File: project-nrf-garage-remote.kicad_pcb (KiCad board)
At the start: 2 copper layers, 34.5 x 27 mm, 9 parts, among them J1 Screw_Terminal_01x02, J2 Screw_Terminal_01x04, Q1 BSS138W, Q2 BSS138W

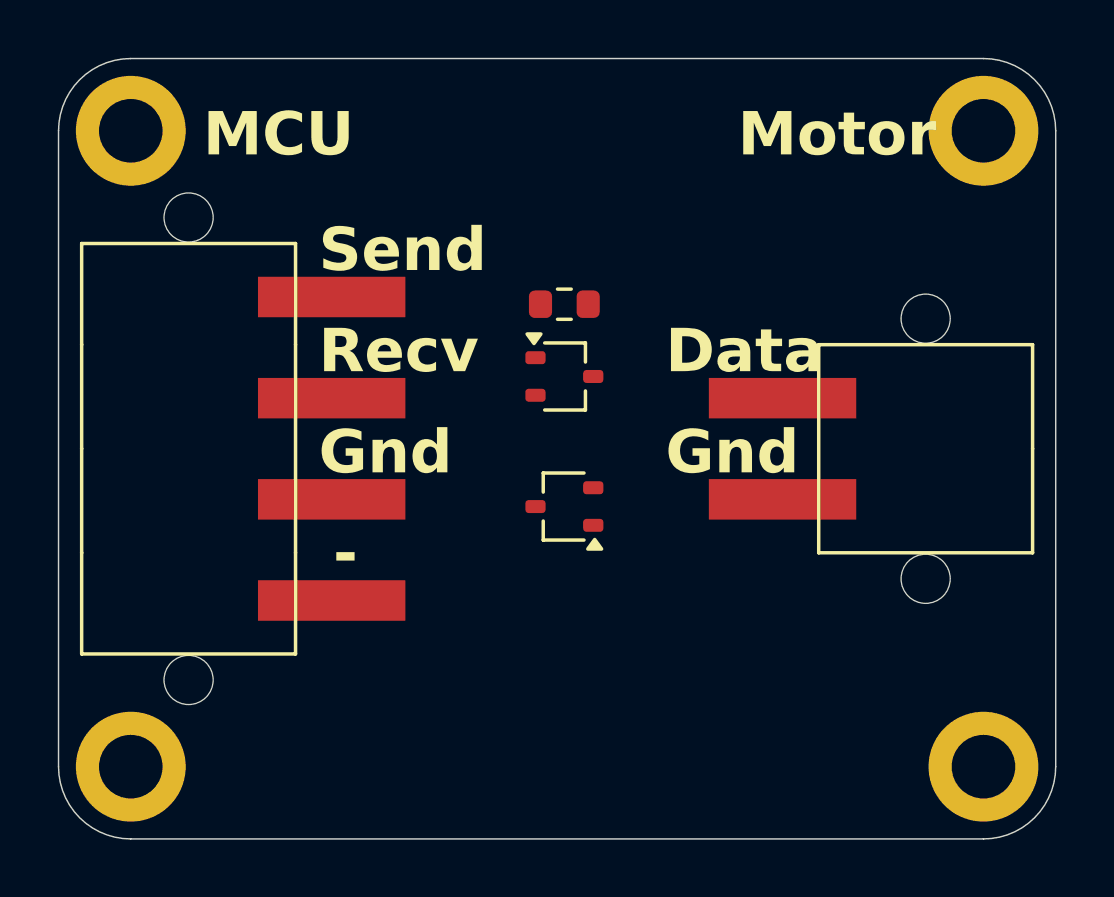
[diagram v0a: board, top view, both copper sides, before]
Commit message: Add routing
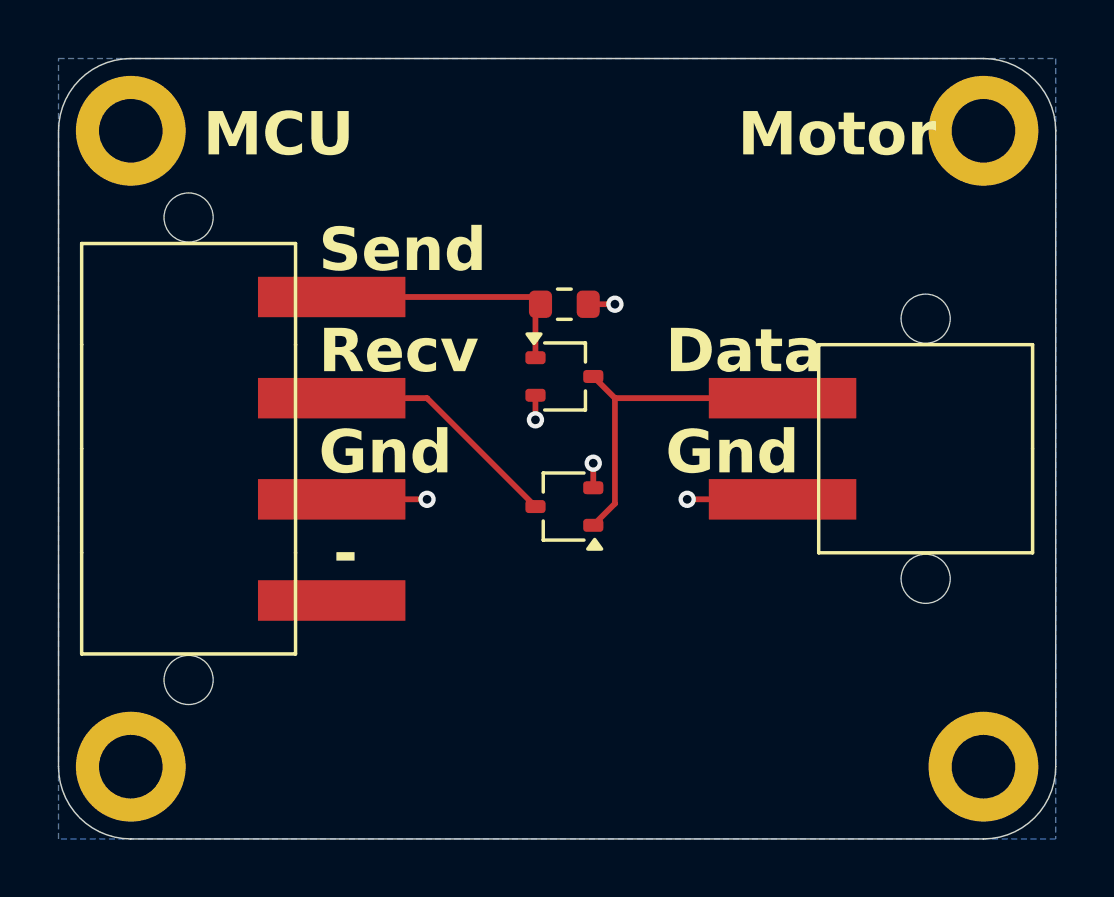
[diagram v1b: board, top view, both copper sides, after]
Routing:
- net /motor_data: track 0.00 -> 11.6 mm
- net /uc_send: track 0.00 -> 9.25 mm
- net GND: track 0.00 -> 9.22 mm, vias 0 -> 5
- net /uc_recv: track 0.00 -> 8.60 mm
- added copper zone on B.Cu, net GND
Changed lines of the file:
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@@
+		)
+	)
+	(segment
+		(start 39.5 29.35)
+		(end 39.5 28.5)
+		(width 0.2)
+		(layer "F.Cu")
+		(net 1)
+	)
+	(segment
+		(start 30.45 29.75)
+		(end 33.75 29.75)
+		(width 0.2)
+		(layer "F.Cu")
+		(net 1)
+	)
+	(segment
+		(start 37.5 26.15)
+		(end 37.5 27)
+		(width 0.2)
+		(layer "F.Cu")
+		(net 1)
+	)
+	(segment
+		(start 39.325 23)
+		(end 40.25 23)
+		(width 0.2)
+		(layer "F.Cu")
+		(net 1)
+	)
+	(segment
+		(start 46.05 29.75)
+		(end 42.75 29.75)
+		(width 0.2)
+		(layer "F.Cu")
+		(net 1)
+	)
+	(via
+		(at 39.5 28.5)
+		(size 0.6)
+		(drill 0.3)
+		(layers "F.Cu" "B.Cu")
+		(net 1)
+	)
+	(via
+		(at 40.25 23)
+		(size 0.6)
+		(drill 0.3)
+		(layers "F.Cu" "B.Cu")
+		(net 1)
+	)
+	(via
+		(at 37.5 27)
+		(size 0.6)
+		(drill 0.3)
+		(layers "F.Cu" "B.Cu")
+		(net 1)
+	)
+	(via
+		(at 33.75 29.75)
+		(size 0.6)
+		(drill 0.3)
+		(layers "F.Cu" "B.Cu")
+		(net 1)
+	)
+	(via
+		(at 42.75 29.75)
+		(size 0.6)
+		(drill 0.3)
+		(layers "F.Cu" "B.Cu")
+		(net 1)
+	)
+	(segment
+		(start 46.05 26.25)
+		(end 40.25 26.25)
+		(width 0.2)
+		(layer "F.Cu")
+		(net 2)
+	)
+	(segment
+		(start 39.5 30.65)
+		(end 40.25 29.9)
+		(width 0.2)
+		(layer "F.Cu")
+		(net 2)
+	)
+	(segment
+		(start 40.25 26.25)
+		(end 39.5 25.5)
+		(width 0.2)
+		(layer "F.Cu")
+		(net 2)
+	)
+	(segment
+		(start 40.25 29.9)
+		(end 40.25 26.25)
+		(width 0.2)
+		(layer "F.Cu")
+		(net 2)
+	)
+	(segment
+		(start 37.5 23.175)
+		(end 37.675 23)
+		(width 0.2)
+		(layer "F.Cu")
+		(net 3)
+	)
+	(segment
+		(start 37.425 22.75)
+		(end 37.675 23)
+		(width 0.2)
+		(layer "F.Cu")
+		(net 3)
+	)
+	(segment
+		(start 30.45 22.75)
+		(end 37.425 22.75)
+		(width 0.2)
+		(layer "F.Cu")
+		(net 3)
+	)
+	(segment
+		(start 37.5 24.85)
+		(end 37.5 23.175)
+		(width 0.2)
+		(layer "F.Cu")
+		(net 3)
+	)
+	(segment
+		(start 33.75 26.25)
+		(end 37.5 30)
+		(width 0.2)
+		(layer "F.Cu")
+		(net 5)
+	)
+	(segment
+		(start 30.45 26.25)
+		(end 33.75 26.25)
+		(width 0.2)
+		(layer "F.Cu")
+		(net 5)
+	)
+	(zone
+		(net 1)
+		(net_name "GND")
+		(layer "B.Cu")
+		(hatch edge 0.5)
+		(connect_pads
+			(clearance 0.5)
+		)
+		(min_thickness 0.25)
+		(filled_areas_thickness no)
+		(fill yes
+			(thermal_gap 0.5)
+			(thermal_bridge_width 0.5)
+		)
+		(polygon
+			(pts
+				(xy 21 41.5) (xy 21 14.5) (xy 55.5 14.5) (xy 55.5 41.5)
+			)
 		)
 	)
